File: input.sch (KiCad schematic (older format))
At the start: 8 parts, among them P20 5V+, P21 5V-, P22 PSU_TERMINAL_BLOCK, P23 SENOSRS_IN, P24 PSU_VIN, P25 PSU_VIN-, SW1 RST

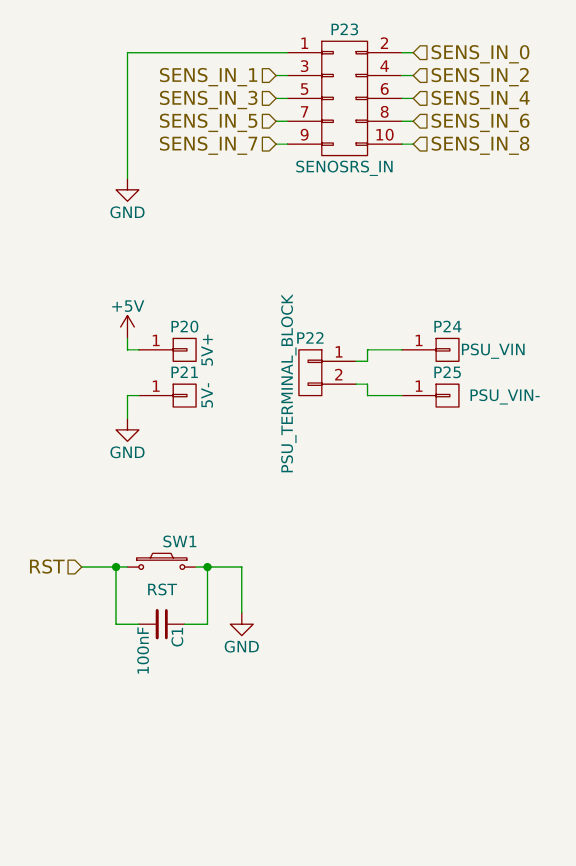
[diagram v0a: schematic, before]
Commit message: PCB rev1.0
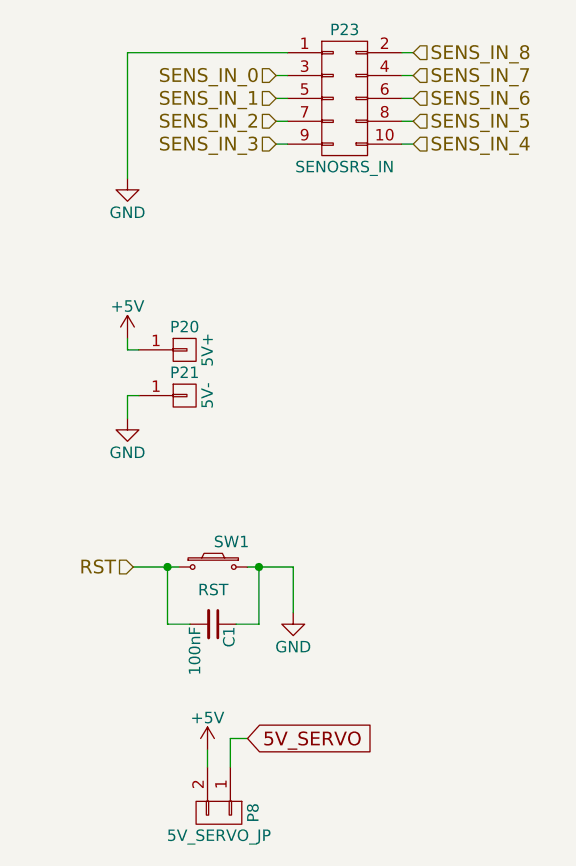
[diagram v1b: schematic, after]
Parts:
- removed P22: PSU_TERMINAL_BLOCK, Pin_Headers:Pin_Header_Straight_1x02, symbol CONN_01X02
- removed P24: PSU_VIN, Pin_Headers:Pin_Header_Straight_1x01, symbol CONN_01X01
- removed P25: PSU_VIN-, Pin_Headers:Pin_Header_Straight_1x01, symbol CONN_01X01
- added P8: 5V_SERVO_JP, Socket_Strips:Socket_Strip_Straight_1x02, symbol CONN_01X02
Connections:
- net +5V: now also P8.2 (P2)
- net SENS_IN_0: now also P23.3 (P3); no longer P23.2 (P2)
- net SENS_IN_1: now also P23.5 (P5); no longer P23.3 (P3)
- net SENS_IN_2: now also P23.7 (P7); no longer P23.4 (P4)
- net SENS_IN_3: now also P23.9 (P9); no longer P23.5 (P5)
- net SENS_IN_4: now also P23.10 (P10); no longer P23.6 (P6)
- net SENS_IN_5: now also P23.8 (P8); no longer P23.7 (P7)
- net SENS_IN_6: now also P23.6 (P6); no longer P23.8 (P8)
- net SENS_IN_7: now also P23.4 (P4); no longer P23.9 (P9)
- net SENS_IN_8: now also P23.2 (P2); no longer P23.10 (P10)
- new net 5V_SERVO: P8.1 (P1)
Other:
- moved on the sheet: C1, SW1
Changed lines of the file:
@@
 $EndComp
 $Comp
-L GND #PWR014
+L GND #PWR010
 U 1 1 57FDABFE
 P 1000 1450
-F 0 "#PWR014" H 1000 1200 50  0001 C CNN
+F 0 "#PWR010" H 1000 1200 50  0001 C CNN
 F 1 "GND" H 1000 1300 50  0000 C CNN
 F 2 "" H 1000 1450 50  0000 C CNN
@@
 Wire Wire Line
 	1000 900  1700 900
+Text HLabel 1650 1100 0    60   Input ~ 0
+SENS_IN_1
+Text HLabel 1650 1300 0    60   Input ~ 0
+SENS_IN_3
+Text HLabel 2250 1200 2    60   Input ~ 0
+SENS_IN_5
+Text HLabel 2250 1000 2    60   Input ~ 0
+SENS_IN_7
 Text HLabel 1650 1000 0    60   Input ~ 0
-SENS_IN_1
-Text HLabel 1650 1100 0    60   Input ~ 0
-SENS_IN_3
+SENS_IN_0
 Text HLabel 1650 1200 0    60   Input ~ 0
-SENS_IN_5
-Text HLabel 1650 1300 0    60   Input ~ 0
-SENS_IN_7
+SENS_IN_2
+Text HLabel 2250 1300 2    60   Input ~ 0
+SENS_IN_4
+Text HLabel 2250 1100 2    60   Input ~ 0
+SENS_IN_6
 Text HLabel 2250 900  2    60   Input ~ 0
-SENS_IN_0
-Text HLabel 2250 1000 2    60   Input ~ 0
-SENS_IN_2
-Text HLabel 2250 1100 2    60   Input ~ 0
-SENS_IN_4
-Text HLabel 2250 1200 2    60   Input ~ 0
-SENS_IN_6
-Text HLabel 2250 1300 2    60   Input ~ 0
 SENS_IN_8
 Wire Wire Line
@@
 $EndComp
 $Comp
-L +5V #PWR015
+L +5V #PWR011
 U 1 1 57FE18D7
 P 1000 2150
-F 0 "#PWR015" H 1000 2000 50  0001 C CNN
+F 0 "#PWR011" H 1000 2000 50  0001 C CNN
 F 1 "+5V" H 1000 2290 50  0000 C CNN
 F 2 "" H 1000 2150 50  0000 C CNN
@@
 $EndComp
 $Comp
-L GND #PWR016
+L GND #PWR012
 U 1 1 57FE1B21
 P 1000 2500
-F 0 "#PWR016" H 1000 2250 50  0001 C CNN
+F 0 "#PWR012" H 1000 2250 50  0001 C CNN
 F 1 "GND" H 1000 2350 50  0000 C CNN
 F 2 "" H 1000 2500 50  0000 C CNN
@@
 	1000 2400 1000 2500
 $Comp
-L CONN_01X01 P24
-U 1 1 57FE1DE8
-P 2400 2200
-F 0 "P24" H 2400 2300 50  0000 C CNN
-F 1 "PSU_VIN" H 2600 2200 50  0000 C CNN
-F 2 "Pin_Headers:Pin_Header_Straight_1x01" H 2400 2200 50  0001 C CNN
-F 3 "" H 2400 2200 50  0000 C CNN
-	1    2400 2200
-	1    0    0    -1
-$EndComp
-$Comp
-L CONN_01X01 P25
-U 1 1 57FE1DF6
-P 2400 2400
-F 0 "P25" H 2400 2500 50  0000 C CNN
-F 1 "PSU_VIN-" H 2650 2400 50  0000 C CNN
-F 2 "Pin_Headers:Pin_Header_Straight_1x01" H 2400 2400 50  0001 C CNN
-F 3 "" H 2400 2400 50  0000 C CNN
-	1    2400 2400
-	1    0    0    -1
-$EndComp
-$Comp
-L CONN_01X02 P22
-U 1 1 57FE2158
-P 1800 2300
-F 0 "P22" H 1800 2450 50  0000 C CNN
-F 1 "PSU_TERMINAL_BLOCK" V 1900 2250 50  0000 C CNN
-F 2 "Pin_Headers:Pin_Header_Straight_1x02" H 1800 2300 50  0001 C CNN
-F 3 "" H 1800 2300 50  0000 C CNN
-	1    1800 2300
-	-1   0    0    -1
-$EndComp
-Wire Wire Line
-	2000 2250 2050 2250
-Wire Wire Line
-	2050 2250 2050 2200
-Wire Wire Line
-	2050 2200 2200 2200
-Wire Wire Line
-	2000 2350 2050 2350
-Wire Wire Line
-	2050 2350 2050 2400
-Wire Wire Line
-	2050 2400 2200 2400
-$Comp
 L SW_PUSH_SMALL_H SW1
 U 1 1 57FE29DD
-P 1150 3150
-F 0 "SW1" H 1230 3260 50  0000 C CNN
-F 1 "RST" H 1150 3050 50  0000 C CNN
-F 2 "Buttons_Switches_SMD:SW_SPST_REED_CT05-XXXX-G1" H 1150 3350 50  0001 C CNN
-F 3 "" H 1150 3350 50  0000 C CNN
-	1    1150 3150
+P 1375 3150
+F 0 "SW1" H 1455 3260 50  0000 C CNN
+F 1 "RST" H 1375 3050 50  0000 C CNN
+F 2 "Buttons_Switches_SMD:SW_SPST_REED_CT05-XXXX-G1" H 1375 3350 50  0001 C CNN
+F 3 "" H 1375 3350 50  0000 C CNN
+	1    1375 3150
 	1    0    0    -1
 $EndComp
@@
 L C_Small C1
 U 1 1 57FE2CD4
-P 1150 3400
-F 0 "C1" H 1160 3470 50  0000 L CNN
-F 1 "100nF" H 1160 3320 50  0000 L CNN
-F 2 "Capacitors_SMD:C_0805_HandSoldering" H 1150 3400 50  0001 C CNN
-F 3 "" H 1150 3400 50  0000 C CNN
-	1    1150 3400
+P 1375 3400
+F 0 "C1" H 1385 3470 50  0000 L CNN
+F 1 "100nF" H 1385 3320 50  0000 L CNN
+F 2 "Capacitors_SMD:C_0805_HandSoldering" H 1375 3400 50  0001 C CNN
+F 3 "" H 1375 3400 50  0000 C CNN
+	1    1375 3400
 	0    1    1    0
 $EndComp
 Wire Wire Line
-	1050 3400 950  3400
+	1275 3400 1175 3400
 Wire Wire Line
-	950  3400 950  3150
+	1175 3400 1175 3150
 Wire Wire Line
-	800  3150 1000 3150
+	1025 3150 1225 3150
 Wire Wire Line
-	1250 3400 1350 3400
+	1475 3400 1575 3400
 Wire Wire Line
-	1350 3400 1350 3150
+	1575 3400 1575 3150
 Wire Wire Line
-	1300 3150 1500 3150
-Text HLabel 800  3150 0    60   Input ~ 0
+	1525 3150 1725 3150
+Text HLabel 1025 3150 0    60   Input ~ 0
 RST
-Connection ~ 950  3150
+Connection ~ 1175 3150
 $Comp
-L GND #PWR017
+L GND #PWR013
 U 1 1 57FE30FD
-P 1500 3350
-F 0 "#PWR017" H 1500 3100 50  0001 C CNN
-F 1 "GND" H 1500 3200 50  0000 C CNN
-F 2 "" H 1500 3350 50  0000 C CNN
-F 3 "" H 1500 3350 50  0000 C CNN
-	1    1500 3350
+P 1725 3350
+F 0 "#PWR013" H 1725 3100 50  0001 C CNN
+F 1 "GND" H 1725 3200 50  0000 C CNN
+F 2 "" H 1725 3350 50  0000 C CNN
+F 3 "" H 1725 3350 50  0000 C CNN
+	1    1725 3350
 	1    0    0    -1
 $EndComp
 Wire Wire Line
-	1500 3150 1500 3350
-Connection ~ 1350 3150
+	1725 3150 1725 3350
+Connection ~ 1575 3150
+$Comp
+L CONN_01X02 P8
+U 1 1 57FEDB28
+P 1400 4225
+F 0 "P8" H 1400 4375 50  0000 C CNN
+F 1 "5V_SERVO_JP" V 1500 4225 50  0000 C CNN
+F 2 "Socket_Strips:Socket_Strip_Straight_1x02" H 1400 4225 50  0001 C CNN
+F 3 "" H 1400 4225 50  0000 C CNN
+	1    1400 4225
+	0    1    1    0
+$EndComp
+$Comp
+L +5V #PWR014
+U 1 1 57FEDDD4
+P 1350 3950
+F 0 "#PWR014" H 1350 3800 50  0001 C CNN
+F 1 "+5V" H 1350 4090 50  0000 C CNN
+F 2 "" H 1350 3950 50  0000 C CNN
+F 3 "" H 1350 3950 50  0000 C CNN
+	1    1350 3950
+	1    0    0    -1
+$EndComp
+Wire Wire Line
+	1350 3950 1350 4025
+Text GLabel 1525 3900 2    60   Input ~ 0
+5V_SERVO
+Wire Wire Line
+	1450 4025 1450 3900
+Wire Wire Line
+	1450 3900 1525 3900
 $EndSCHEMATC

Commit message: pcb rev2
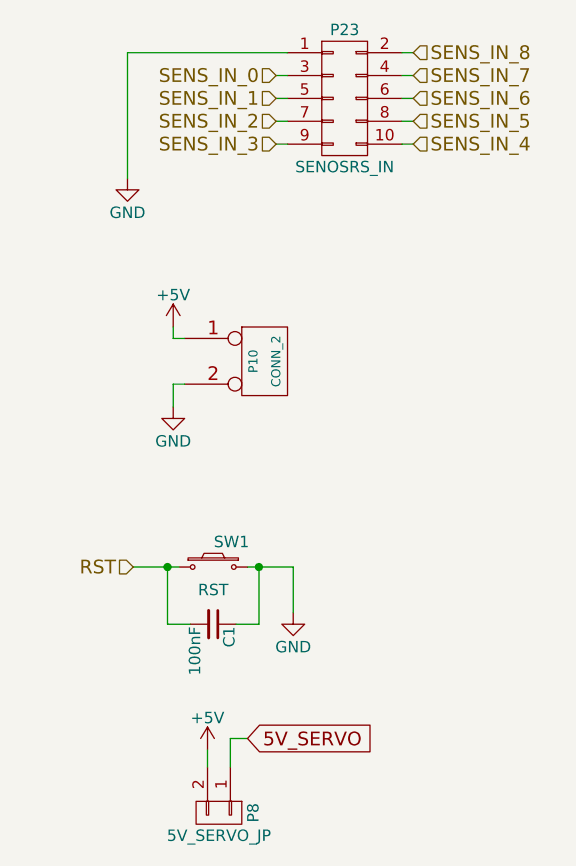
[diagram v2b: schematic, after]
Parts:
- removed P20: 5V+, Pin_Headers:Pin_Header_Straight_1x01, symbol CONN_01X01
- removed P21: 5V-, Pin_Headers:Pin_Header_Straight_1x01, symbol CONN_01X01
- added P10: CONN_2, Terminal_Blocks:TerminalBlock_Pheonix_MKDS1.5-2pol, symbol CONN_2
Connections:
- net +5V: now also P10.1 (P1)
- net GND: now also P10.2 (P2)
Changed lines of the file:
@@
 LIBS:contrib
 LIBS:valves
+LIBS:borniers
 LIBS:Arduino_Mega-cache
 EELAYER 25 0
@@
 	2200 900  2250 900
 $Comp
-L CONN_01X01 P20
-U 1 1 57FE1867
-P 1250 2200
-F 0 "P20" H 1250 2300 50  0000 C CNN
-F 1 "5V+" V 1350 2200 50  0000 C CNN
-F 2 "Pin_Headers:Pin_Header_Straight_1x01" H 1250 2200 50  0001 C CNN
-F 3 "" H 1250 2200 50  0000 C CNN
-	1    1250 2200
-	1    0    0    -1
-$EndComp
-$Comp
 L +5V #PWR011
 U 1 1 57FE18D7
-P 1000 2150
-F 0 "#PWR011" H 1000 2000 50  0001 C CNN
-F 1 "+5V" H 1000 2290 50  0000 C CNN
-F 2 "" H 1000 2150 50  0000 C CNN
-F 3 "" H 1000 2150 50  0000 C CNN
-	1    1000 2150
-	1    0    0    -1
-$EndComp
-Wire Wire Line
-	1000 2150 1000 2200
-Wire Wire Line
-	1000 2200 1050 2200
-$Comp
-L CONN_01X01 P21
-U 1 1 57FE1ADE
-P 1250 2400
-F 0 "P21" H 1250 2500 50  0000 C CNN
-F 1 "5V-" V 1350 2400 50  0000 C CNN
-F 2 "Pin_Headers:Pin_Header_Straight_1x01" H 1250 2400 50  0001 C CNN
-F 3 "" H 1250 2400 50  0000 C CNN
-	1    1250 2400
-	1    0    0    -1
-$EndComp
+P 1200 2100
+F 0 "#PWR011" H 1200 1950 50  0001 C CNN
+F 1 "+5V" H 1200 2240 50  0000 C CNN
+F 2 "" H 1200 2100 50  0000 C CNN
+F 3 "" H 1200 2100 50  0000 C CNN
+	1    1200 2100
+	1    0    0    -1
+$EndComp
+Wire Wire Line
+	1200 2100 1200 2150
+Wire Wire Line
+	1200 2150 1250 2150
 $Comp
 L GND #PWR012
 U 1 1 57FE1B21
-P 1000 2500
-F 0 "#PWR012" H 1000 2250 50  0001 C CNN
-F 1 "GND" H 1000 2350 50  0000 C CNN
-F 2 "" H 1000 2500 50  0000 C CNN
-F 3 "" H 1000 2500 50  0000 C CNN
-	1    1000 2500
-	1    0    0    -1
-$EndComp
-Wire Wire Line
-	1050 2400 1000 2400
-Wire Wire Line
-	1000 2400 1000 2500
+P 1200 2450
+F 0 "#PWR012" H 1200 2200 50  0001 C CNN
+F 1 "GND" H 1200 2300 50  0000 C CNN
+F 2 "" H 1200 2450 50  0000 C CNN
+F 3 "" H 1200 2450 50  0000 C CNN
+	1    1200 2450
+	1    0    0    -1
+$EndComp
+Wire Wire Line
+	1250 2350 1200 2350
+Wire Wire Line
+	1200 2350 1200 2450
 $Comp
 L SW_PUSH_SMALL_H SW1
@@
 Wire Wire Line
 	1450 3900 1525 3900
+$Comp
+L CONN_2 P10
+U 1 1 57FFF850
+P 1600 2250
+F 0 "P10" V 1550 2250 40  0000 C CNN
+F 1 "CONN_2" V 1650 2250 40  0000 C CNN
+F 2 "Terminal_Blocks:TerminalBlock_Pheonix_MKDS1.5-2pol" H 1600 2250 60  0001 C CNN
+F 3 "" H 1600 2250 60  0001 C CNN
+	1    1600 2250
+	1    0    0    -1
+$EndComp
 $EndSCHEMATC
